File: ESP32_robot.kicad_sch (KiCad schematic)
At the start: 30 parts, among them J1 USB_C_Receptacle_USB2.0, J2 Conn_01x08_Male, J3 01x02, J4 Conn_01x08_Male, J5 01x02, SW1 SW_Push, SW2 SW_Push, U1 ESP32-S2-MINI-1-N4, U2 LM1117-3.3

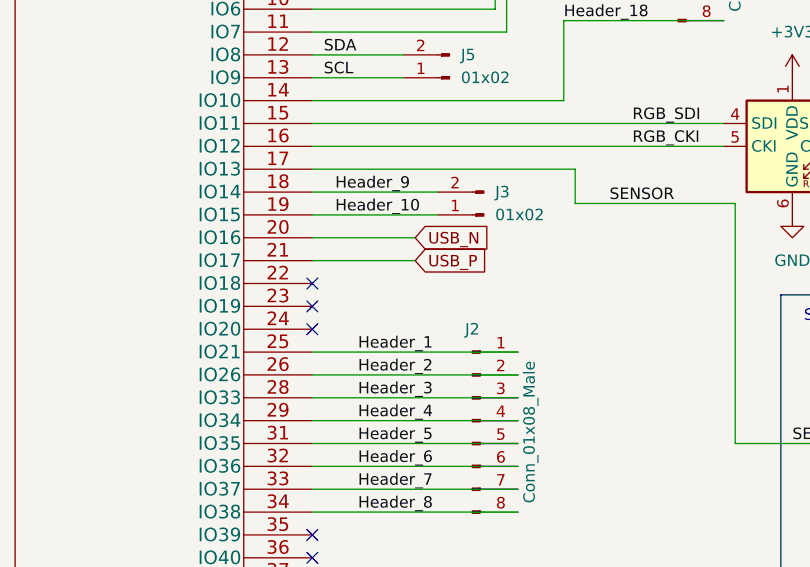
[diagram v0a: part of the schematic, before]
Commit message: hopefully the latest
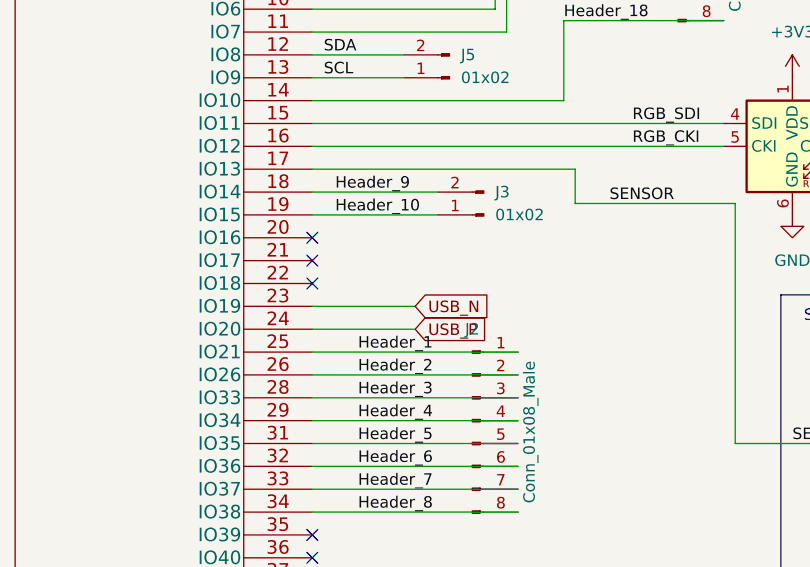
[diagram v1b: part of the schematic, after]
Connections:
- net USB_N: now also U1.23 (IO19); no longer U1.20 (IO16)
- net USB_P: now also U1.24 (IO20); no longer U1.21 (IO17)
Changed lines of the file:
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@@
   (junction (at 248.92 72.39) (diameter 0) (color 0 0 0 0)
   )
-  (no_connect (at 66.04 144.78))
-  (no_connect (at 66.04 147.32))
+  (no_connect (at 66.04 139.7))
+  (no_connect (at 66.04 137.16))
   (no_connect (at 25.4 99.06))
   (no_connect (at 25.4 101.6))
@@
     (stroke (width 0) (type default) (color 0 0 0 0))
   )
-  (wire (pts (xy 66.04 139.7) (xy 77.47 139.7))
+  (wire (pts (xy 66.04 147.32) (xy 77.47 147.32))
     (stroke (width 0) (type default) (color 0 0 0 0))
   )
@@
     (stroke (width 0) (type default) (color 0 0 0 0))
   )
-  (wire (pts (xy 66.04 137.16) (xy 77.47 137.16))
+  (wire (pts (xy 66.04 144.78) (xy 77.47 144.78))
     (stroke (width 0) (type default) (color 0 0 0 0))
   )
@@
     )
   )
-  (global_label "USB_P" (shape input) (at 77.47 139.7 0) (fields_autoplaced)
+  (global_label "USB_P" (shape input) (at 77.47 147.32 0) (fields_autoplaced)
     (effects (font (size 1.27 1.27)) (justify left))
-    (property "Intersheet References" "${INTERSHEET_REFS}" (id 0) (at 85.9307 139.6206 0)
+    (property "Intersheet References" "${INTERSHEET_REFS}" (id 0) (at 85.9307 147.2406 0)
       (effects (font (size 1.27 1.27)) (justify left) hide)
     )
@@
     )
   )
-  (global_label "USB_N" (shape input) (at 77.47 137.16 0) (fields_autoplaced)
+  (global_label "USB_N" (shape input) (at 77.47 144.78 0) (fields_autoplaced)
     (effects (font (size 1.27 1.27)) (justify left))
-    (property "Intersheet References" "${INTERSHEET_REFS}" (id 0) (at 85.9912 137.0806 0)
+    (property "Intersheet References" "${INTERSHEET_REFS}" (id 0) (at 85.9912 144.7006 0)
       (effects (font (size 1.27 1.27)) (justify left) hide)
     )
@@
     (pin "8")
     (pin "9")
+    (pin "1")
+    (pin "2")
+    (pin "27")
+    (pin "30")
+    (pin "42")
+    (pin "43")
+    (pin "46")
+    (pin "47")
+    (pin "48")
+    (pin "49")
+    (pin "50")
+    (pin "51")
+    (pin "52")
+    (pin "53")
+    (pin "54")
+    (pin "55")
+    (pin "56")
+    (pin "57")
+    (pin "58")
+    (pin "59")
+    (pin "60")
+    (pin "61")
+    (pin "62")
+    (pin "63")
+    (pin "64")
+    (pin "65")
+    (pin "66")
+    (pin "67")
+    (pin "68")
+    (pin "69")
+    (pin "70")
+    (pin "71")
+    (pin "72")
+    (pin "73")
   )
   (symbol (lib_id "power:+3V3") (at 100.33 22.86 0) (unit 1)
@@
       (effects (font (size 1.524 1.524)))
     )
-    (pin "1")
-    (pin "2")
+    (pin "10")
+    (pin "11")
+    (pin "12")
+    (pin "13")
+    (pin "14")
+    (pin "15")
+    (pin "16")
+    (pin "17")
+    (pin "18")
+    (pin "19")
+    (pin "20")
+    (pin "21")
+    (pin "22")
+    (pin "23")
+    (pin "24")
+    (pin "25")
+    (pin "26")
+    (pin "28")
+    (pin "29")
+    (pin "3")
+    (pin "31")
+    (pin "32")
+    (pin "33")
+    (pin "34")
+    (pin "35")
+    (pin "36")
+    (pin "37")
+    (pin "38")
+    (pin "39")
+    (pin "4")
+    (pin "40")
+    (pin "41")
+    (pin "44")
+    (pin "45")
+    (pin "5")
+    (pin "6")
+    (pin "7")
+    (pin "8")
+    (pin "9")
+    (pin "1")
+    (pin "2")
